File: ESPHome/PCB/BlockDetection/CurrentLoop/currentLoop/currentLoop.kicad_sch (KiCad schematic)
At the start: 11 parts, among them J1 Conn_01x03_Pin, J2 Conn_01x02_Pin, J3 Conn_01x02_Pin, Q1 BC856, Q2 BC557, U1 PC817

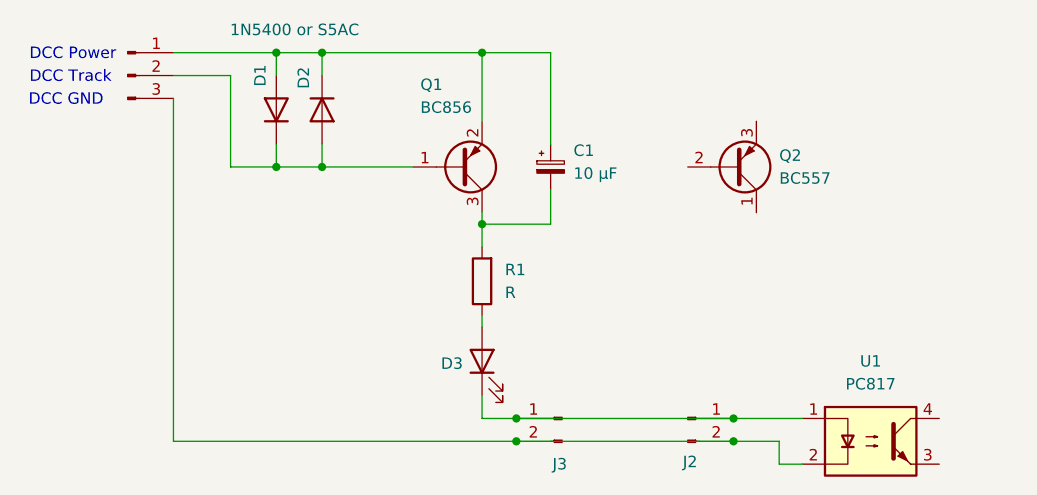
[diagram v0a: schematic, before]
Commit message: current loop
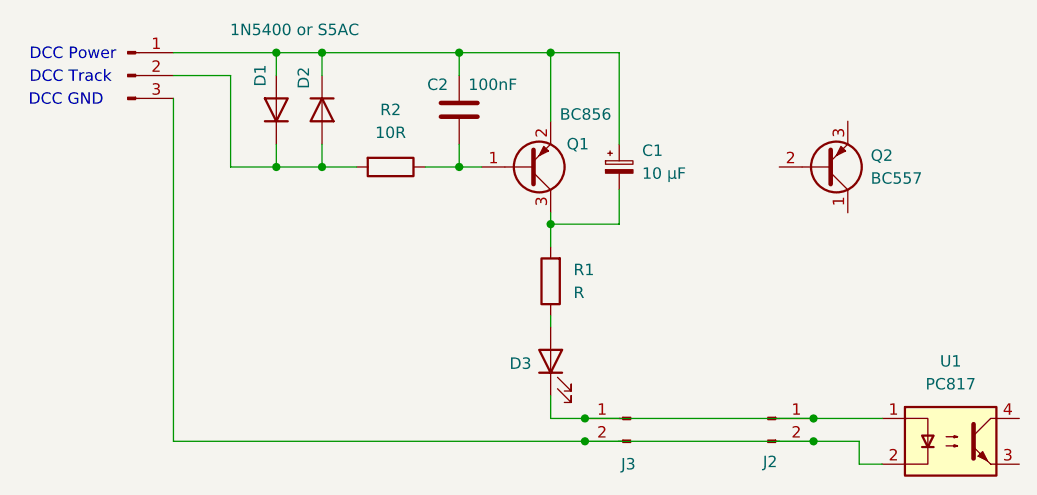
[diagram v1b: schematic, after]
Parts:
- added C2: 100nF, symbol Device:C
- added R2: 10R, symbol Device:R
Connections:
- net at C1.1, D1.2 (A), D2.1 (K)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: now also C2.1
- net at D1.1 (K), D2.2 (A), J1.2 (Pin_2): now also R2.2; no longer Q1.1 (B)
- new net: C2.2, Q1.1 (B), R2.1
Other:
- moved on the sheet: C1, D3, J2, J3, Q1, Q2, R1, U1
